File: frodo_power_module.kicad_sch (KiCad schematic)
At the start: 78 parts, among them J1 Keystone 1098, J10 SWD Header, J2 Molex MicroFit 2x2, J3 Molex MicroFit 2x2, J4 Molex MicroFit 2x2, J5 Molex MicroFit 2x2, J6 Molex MicroFit 2x2, J7 JST-GH, J8 JST-GH, U1 STM32F042F6Px, U2 L7805, U3 AZ1117I-3.3, U4 BQ25171-Q1, U5 BQ29200, U6 MCP2562-E-SN, U7 INA213, Y1 8MHz, 12p

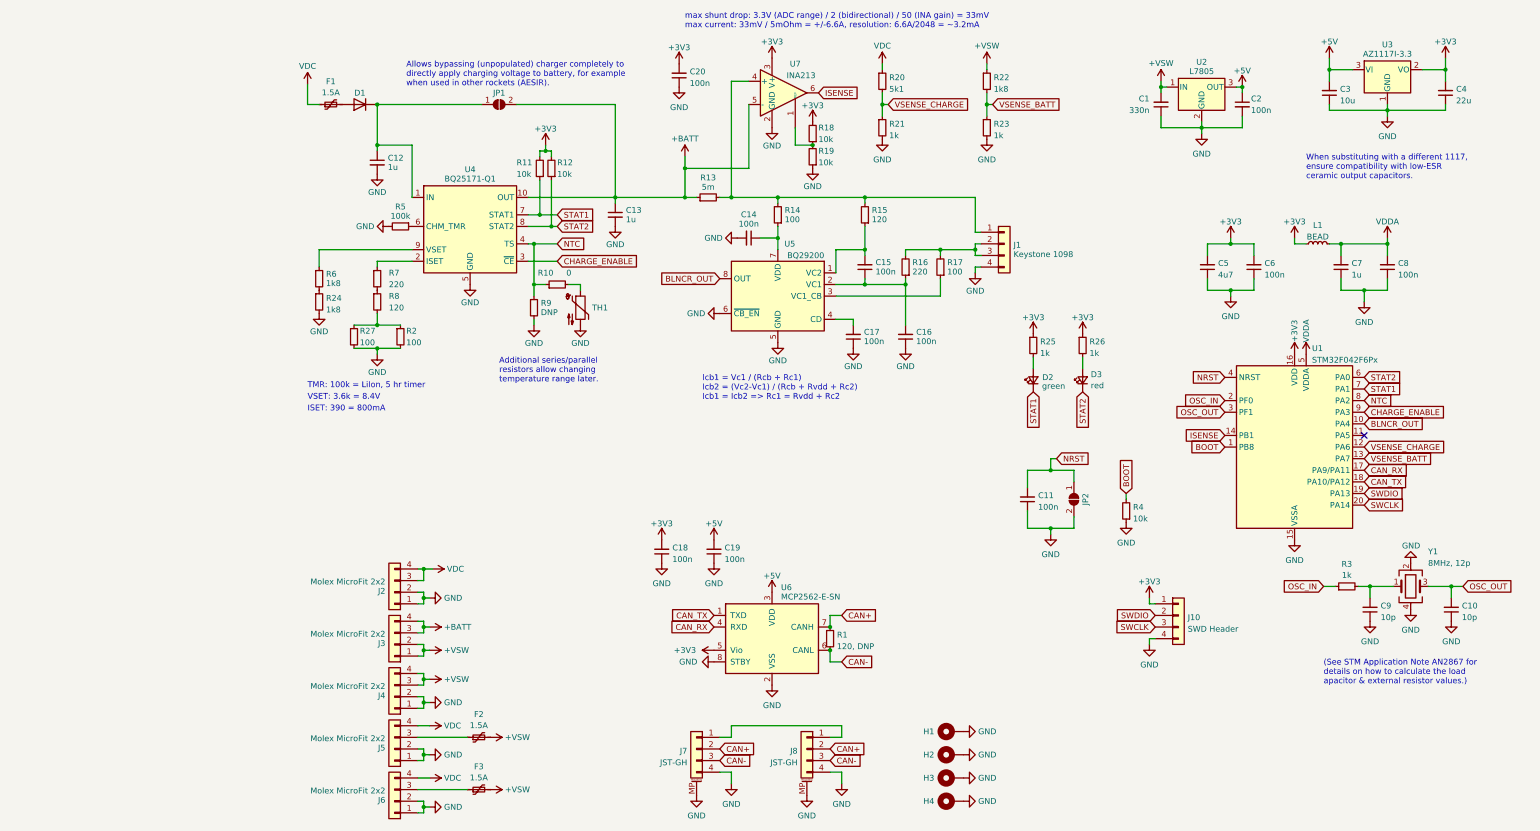
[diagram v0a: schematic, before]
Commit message: modified schematic
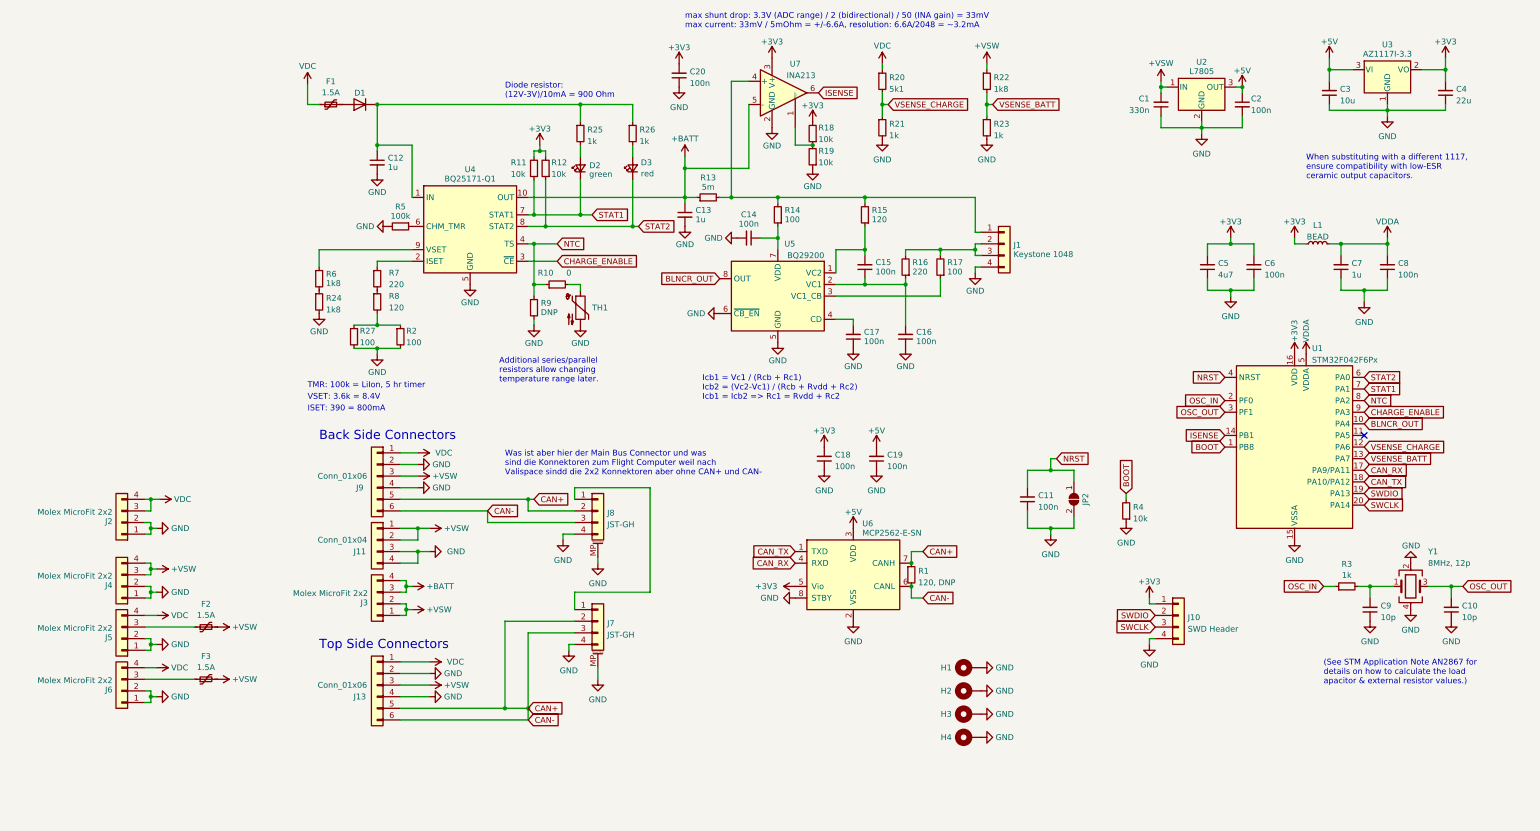
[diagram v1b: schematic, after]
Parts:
- removed JP1: SolderJumper_2_Open, Jumper:SolderJumper-2_P1.3mm_Open_RoundedPad1.0x1.5mm, symbol Jumper:SolderJumper_2_Open
- added J11: Conn_01x04, symbol Connector_Generic:Conn_01x04
- added J13, J9: Conn_01x06, symbol Connector_Generic:Conn_01x06
- J1: value Keystone 1098 -> Keystone 1048; footprint frodo_power_module:keystone_1098 -> frodo_power_module:keystone_1048; Part# 1098 -> 1048
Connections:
- net CAN- is gone; now on net CAN+: J7.3 (Pin_3), J8.3 (Pin_3), R1.2, U6.6 (CANL)
- net +3V3: no longer R25.1, R26.1
- net +VSW: now also J11.1 (Pin_1), J11.2 (Pin_2), J13.3 (Pin_3), J9.3 (Pin_3)
- net CAN+: now also J13.5 (Pin_5), J13.6 (Pin_6), J9.5 (Pin_5), J9.6 (Pin_6)
- net GND: now also J11.3 (Pin_3), J11.4 (Pin_4), J13.2 (Pin_2), J13.4 (Pin_4), J9.2 (Pin_2), J9.4 (Pin_4)
- net VDC: now also J13.1 (Pin_1), J9.1 (Pin_1)
- net at C12.1, D1.1 (K), U4.1 (IN): now also R25.1, R26.1
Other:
- note added: "Back Side Connectors"
- note added: "Diode resistor: (12V-3V)/10mA = 900 Ohm"
- note added: "Top Side Connectors"
- note added: "Was ist aber hier der Main Bus Connector und was sind die Konnektoren zum Flight Computer weil nach Valispace sindd die 2x2 Konnektoren aber ohne CAN+ und CAN-"
- note removed: "Allows bypassing (unpopulated) charger completely to directly apply charging voltage to battery, for example when used in other rockets (AESIR)."
- moved on the sheet: C13, C18, C19, D2, D3, F2, F3, H1, H2, H3, H4, J2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
